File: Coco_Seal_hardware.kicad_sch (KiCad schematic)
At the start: 10 parts, among them P1 USB_C_Plug_USB2.0, SW1 SW_Push_Dual, U1 ESP32-C3-WROOM-02-N4, U2 E220-900T22S（JP）-EV2, U3 ESP32-C3-WROOM-02, U4 ER_OLEDM0.91_1x-I2C, U5 TPSM53602RDA, U6 TP4056-42-ESOP8

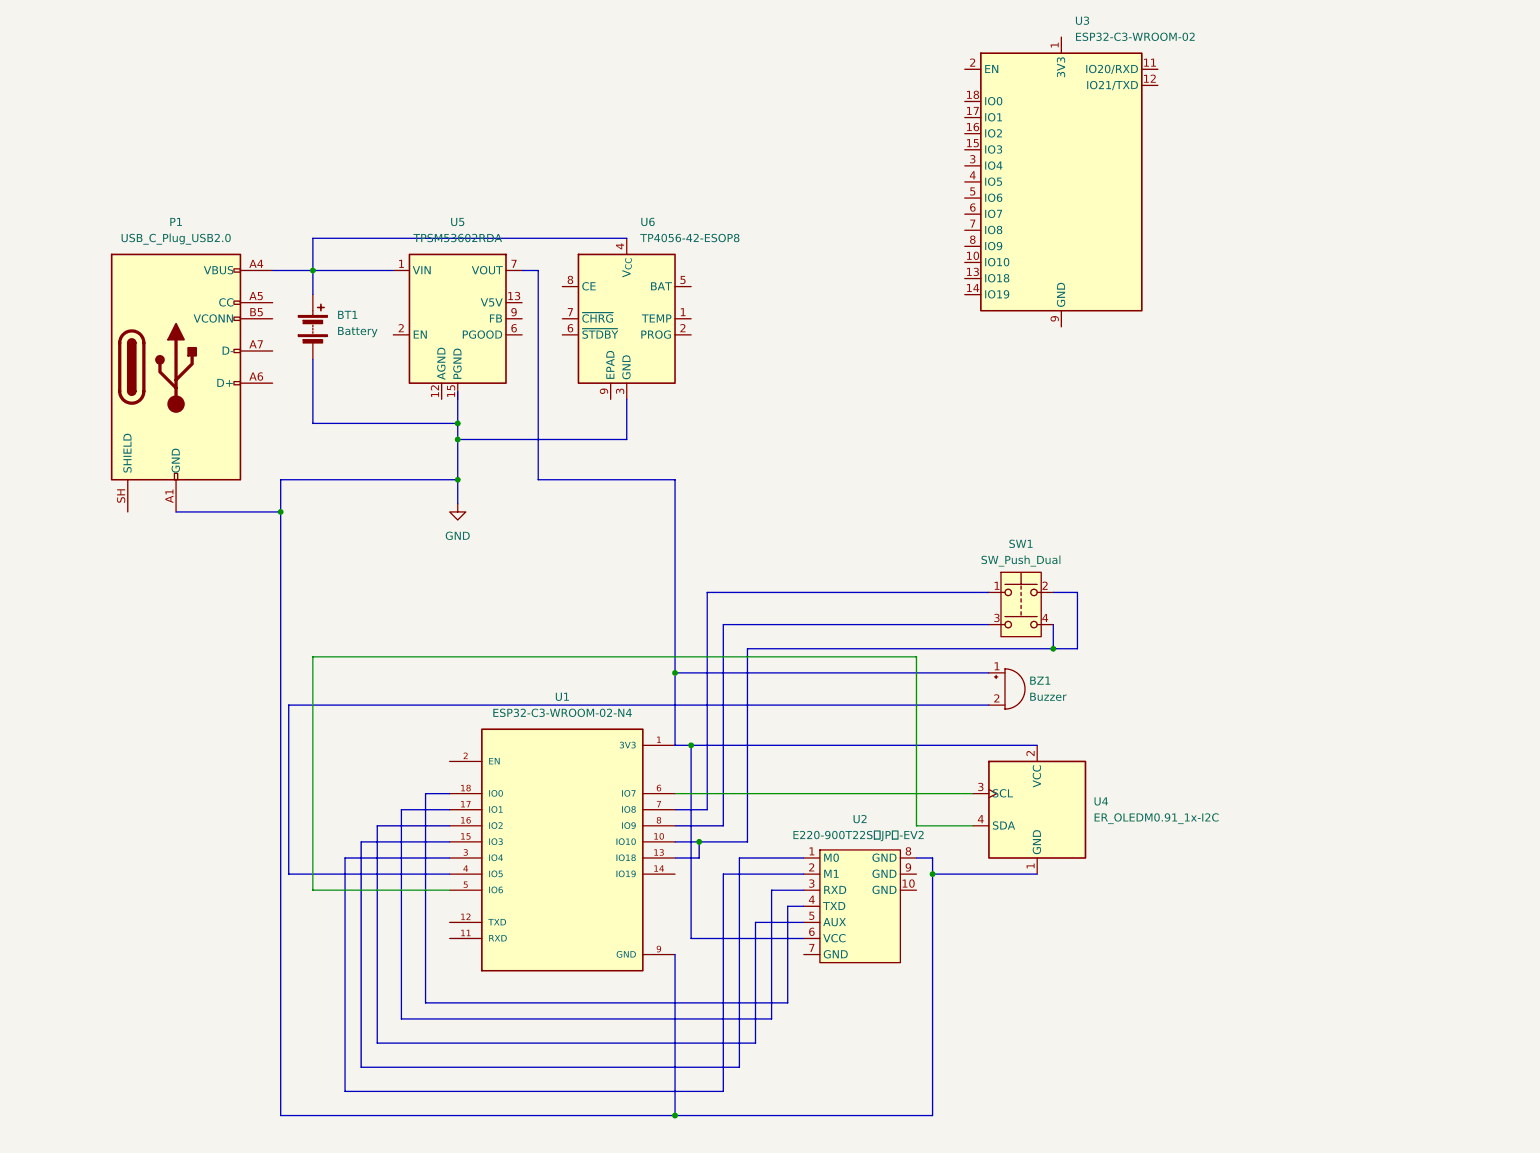
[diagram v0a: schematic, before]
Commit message: README更新, 回路図更新
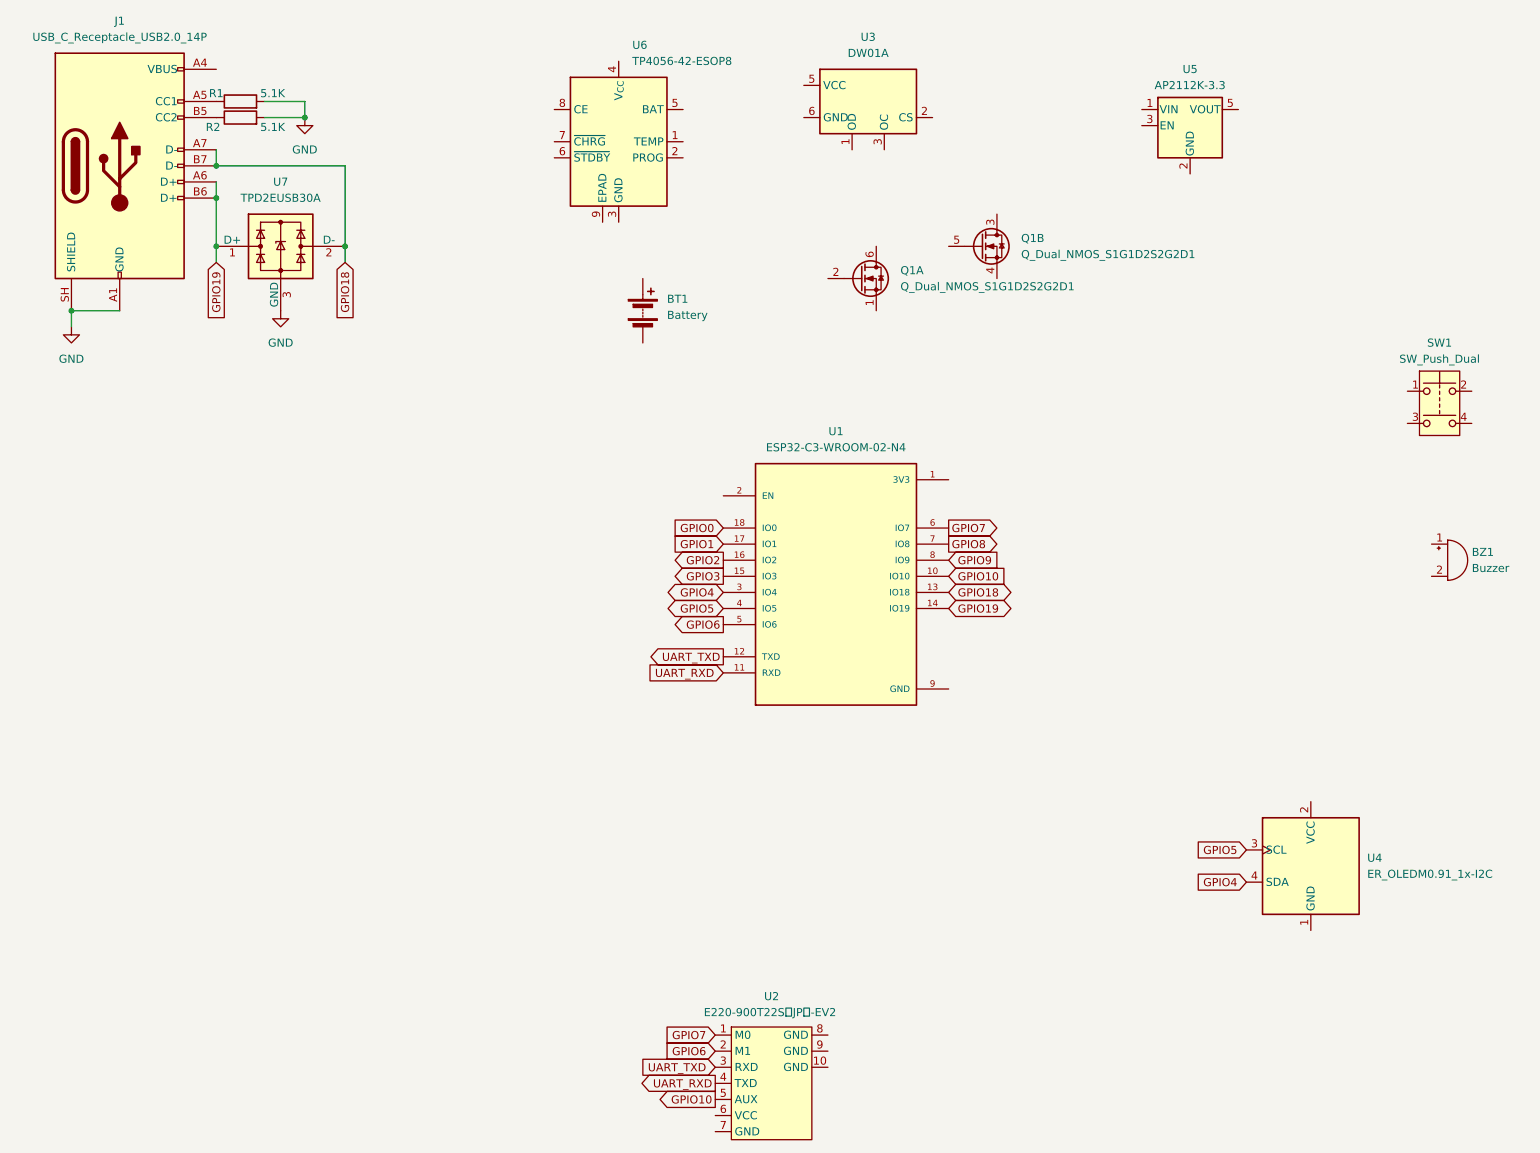
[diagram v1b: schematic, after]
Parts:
- removed P1: USB_C_Plug_USB2.0, symbol Connector:USB_C_Plug_USB2.0
- removed U3: ESP32-C3-WROOM-02, RF_Module:ESP32-C3-WROOM-02, symbol RF_Module:ESP32-C3-WROOM-02
- removed U5: TPSM53602RDA, Package_DFN_QFN:Texas_B3QFN-14-1EP_5x5.5mm_P0.65mm_ThermalVia, symbol Converter_DCDC:TPSM53602RDA
- added J1: USB_C_Receptacle_USB2.0_14P, symbol Connector:USB_C_Receptacle_USB2.0_14P
- added Q1: Q_Dual_NMOS_S1G1D2S2G2D1, Package_TO_SOT_SMD:SOT-23-6, symbol Transistor_FET:Q_Dual_NMOS_S1G1D2S2G2D1
- added R1, R2: 5.1K, symbol Device:R
- added U3: DW01A, Package_TO_SOT_SMD:SOT-23-6, symbol Battery_Management:DW01A
- added U5: AP2112K-3.3, Package_TO_SOT_SMD:SOT-23-5, symbol Regulator_Linear:AP2112K-3.3
- added U7: TPD2EUSB30A, Package_TO_SOT_SMD:Texas_DRT-3, symbol Power_Protection:TPD2EUSB30A
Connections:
- net GND: now also J1.A1 (GND), J1.A12 (GND), J1.B1 (GND), J1.B12 (GND), J1.SH (SHIELD), R1.2, R2.2, U7.3 (GND)
- net GPIO10: now reaches U1.10 (IO10)
- net GPIO10: now also U2.5 (AUX)
- net UART_RXD: now reaches U1.11 (RXD)
- net UART_RXD: now also U2.4 (TXD)
- net UART_TXD: now reaches U1.12 (TXD)
- net UART_TXD: now also U2.3 (RXD)
- net GPIO18: now reaches U1.13 (IO18)
- net GPIO18: now also J1.A7 (D-), J1.B7 (D-), U7.2 (D-)
- net GPIO19: now reaches U1.14 (IO19)
- net GPIO19: now also J1.A6 (D+), J1.B6 (D+), U7.1 (D+)
- net GPIO3: now reaches U1.15 (IO3)
- net GPIO2: now reaches U1.16 (IO2)
- net GPIO1: now reaches U1.17 (IO1)
- net GPIO0: now reaches U1.18 (IO0)
- net GPIO4: now reaches U1.3 (IO4)
- net GPIO4: now also U4.4 (SDA)
- net GPIO5: now reaches U1.4 (IO5)
- net GPIO5: now also U4.3 (SCL)
- net GPIO6: now reaches U1.5 (IO6)
- net GPIO6: now also U2.2 (M1); no longer U4.4 (SDA)
- net GPIO7: now reaches U1.6 (IO7)
- net GPIO7: now also U2.1 (M0); no longer U4.3 (SCL)
- net GPIO8: now reaches U1.7 (IO8)
- net GPIO9: now reaches U1.8 (IO9)
- new net: J1.A4 (VBUS), J1.A9 (VBUS), J1.B4 (VBUS), J1.B9 (VBUS)
- new net: J1.A5 (CC1), R1.1
- new net: J1.B5 (CC2), R2.1
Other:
- moved on the sheet: BT1, BZ1, SW1, U1, U2, U4, U6

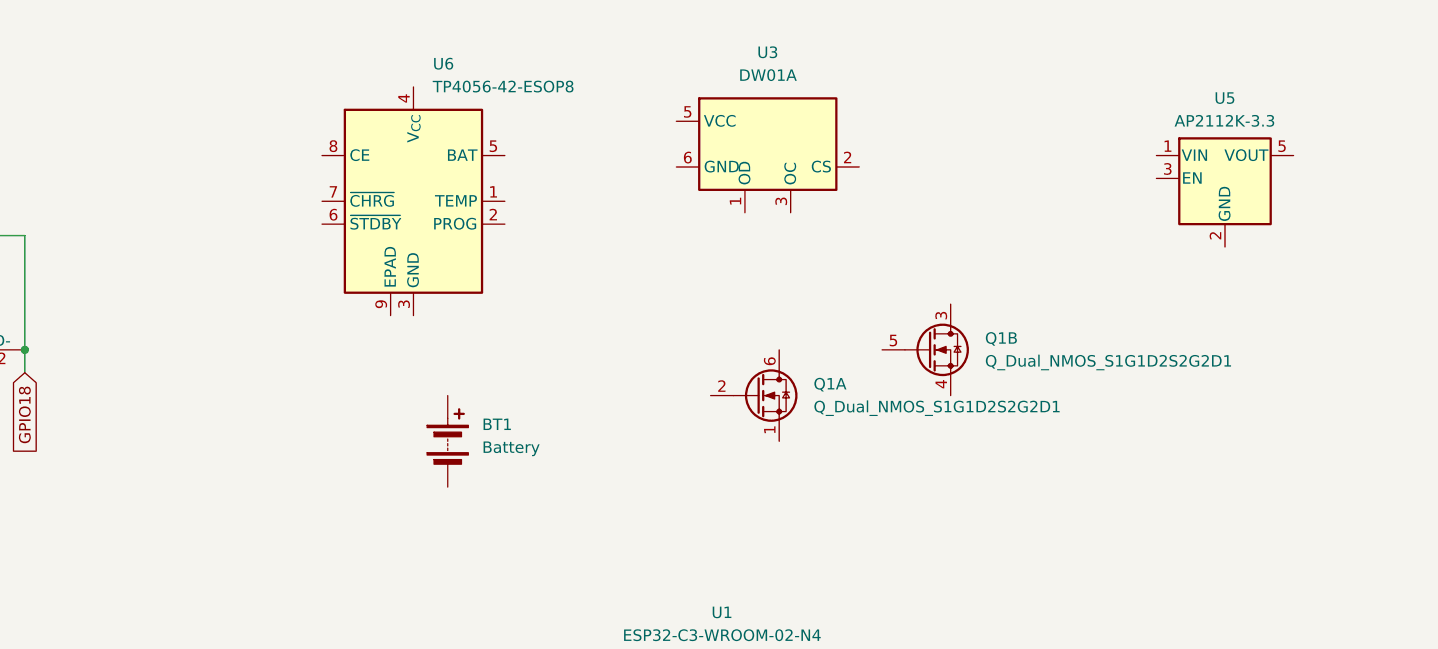
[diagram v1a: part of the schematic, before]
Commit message: 保護回路
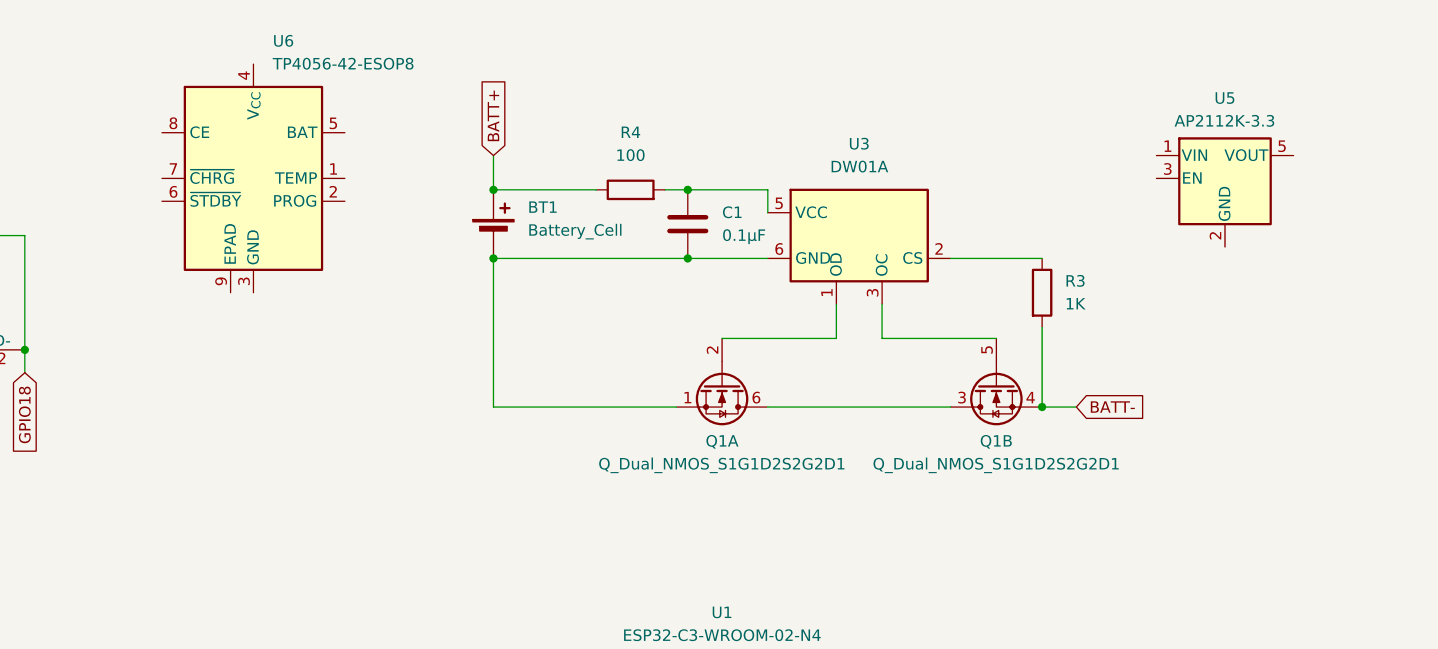
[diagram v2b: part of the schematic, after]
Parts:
- removed BT1: Battery, symbol Device:Battery
- added BT1: Battery_Cell, symbol Device:Battery_Cell
- added C1: 0.1μF, symbol Device:C
- added R3: 1K, symbol Device:R
- added R4: 100, symbol Device:R
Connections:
- net at Q1.1 (S): now also U3.6 (GND), BT1.2 (-), C1.2
- net at Q1.2 (G): now also U3.1 (OD)
- net at Q1.6 (D): now also Q1.3 (D)
- net BATT-: now reaches Q1.4 (S)
- net BATT-: now also R3.2
- net at Q1.5 (G): now also U3.3 (OC)
- net at U3.2 (CS): now also R3.1
- net at U3.5 (VCC): now also C1.1, R4.2
- new net BATT+: BT1.1 (+), R4.1
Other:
- moved on the sheet: Q1A, Q1B, U3, U6
